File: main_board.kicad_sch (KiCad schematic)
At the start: 21 parts, among them SW1 SW_Push, SW2 SW_Push, U4 QM_XC7A35T_DDR3, U8 XLH536074.250000I

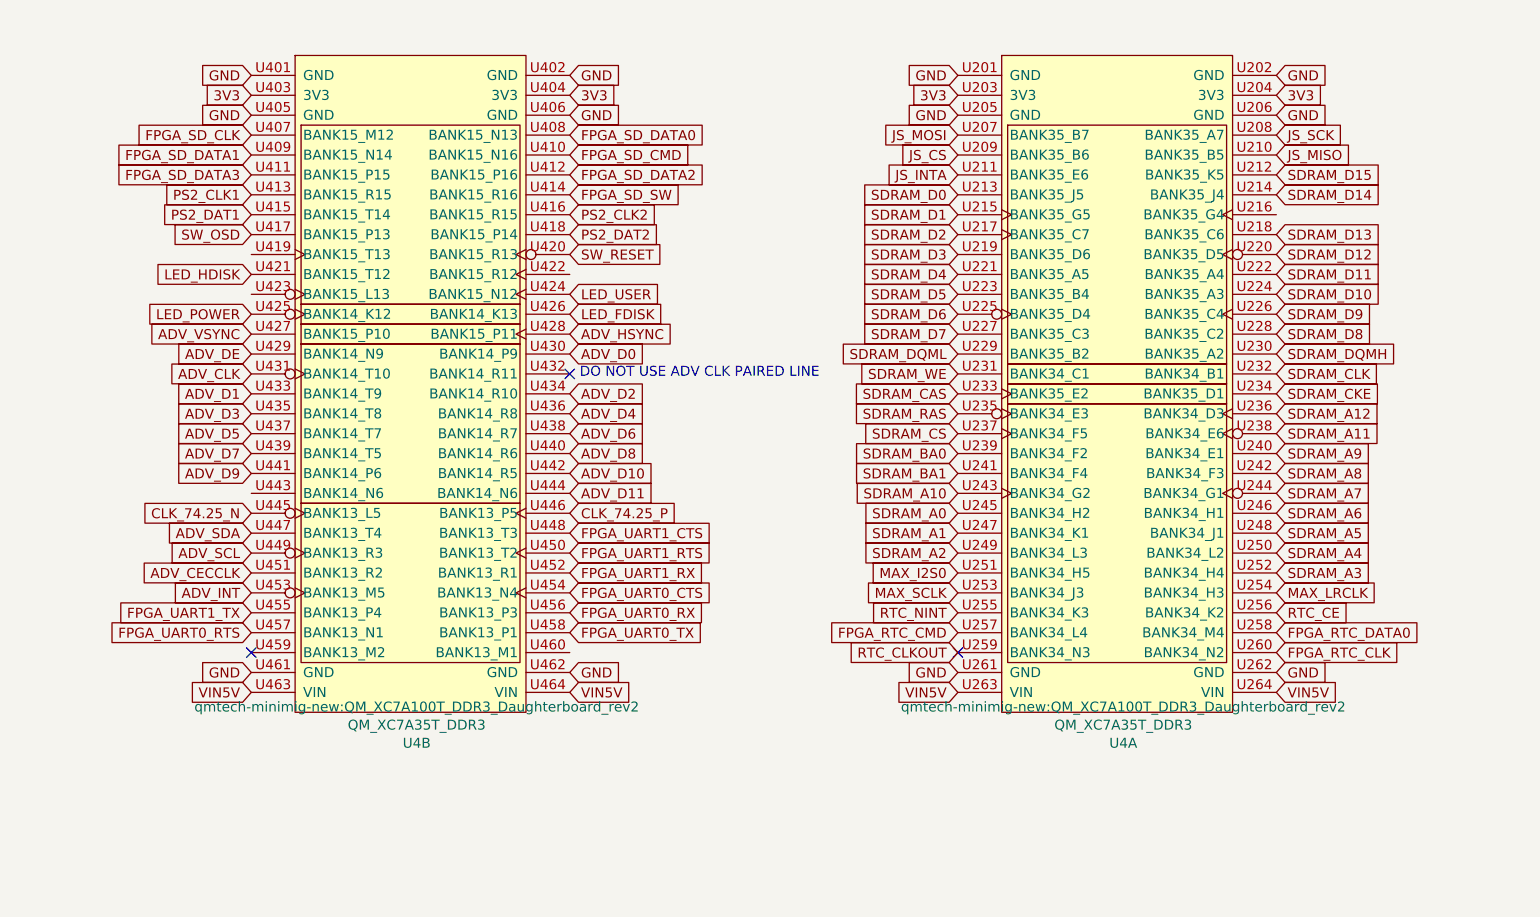
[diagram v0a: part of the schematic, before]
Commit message: V5 Version of the board.
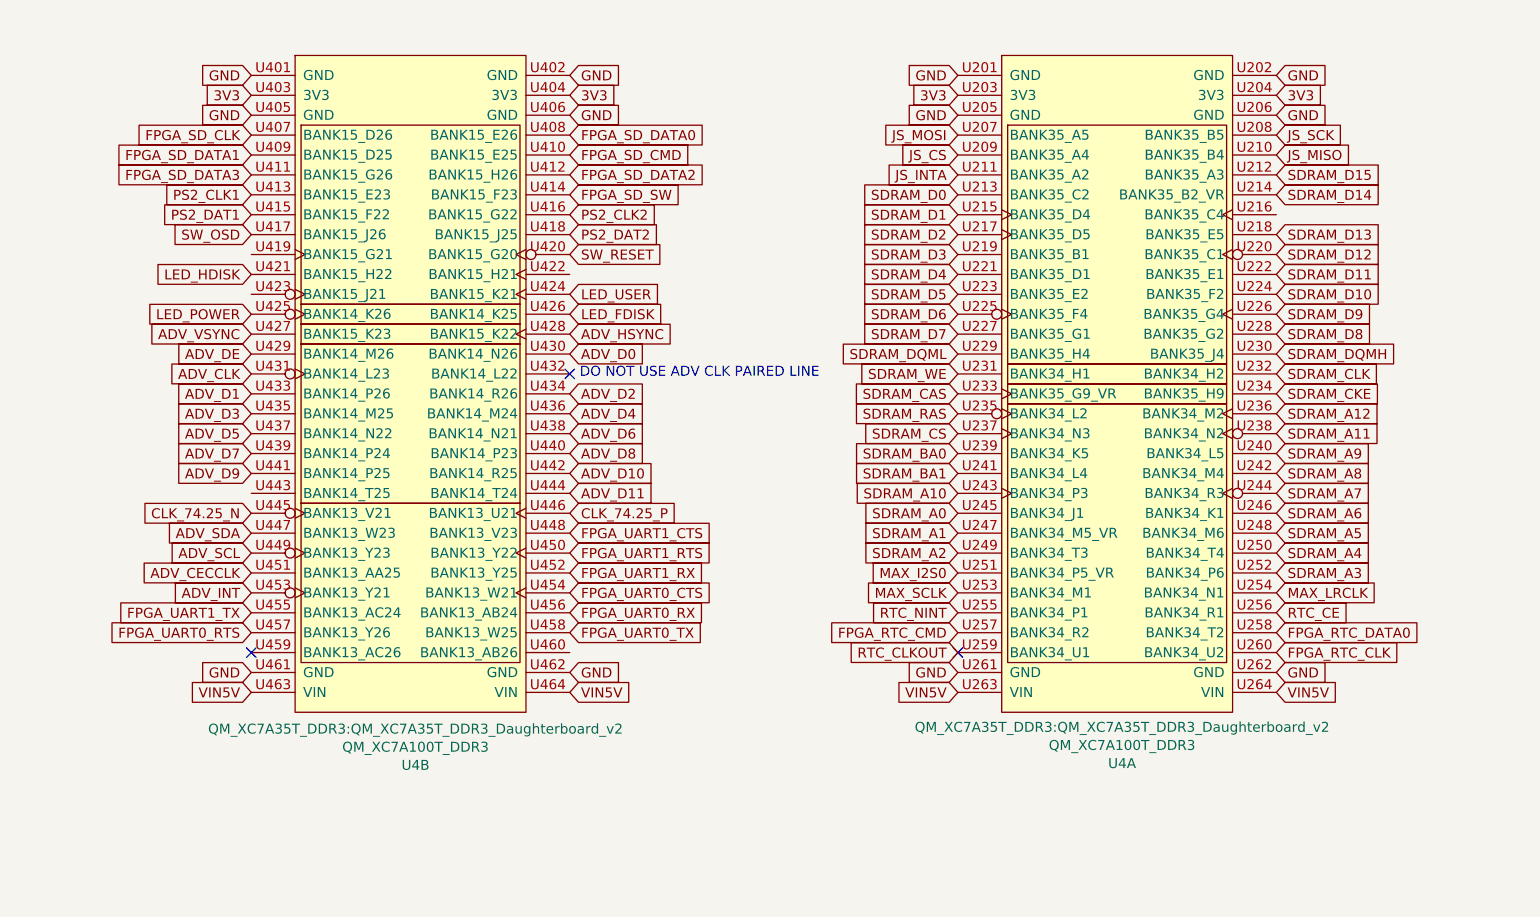
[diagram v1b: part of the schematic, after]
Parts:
- U4: value QM_XC7A35T_DDR3 -> QM_XC7A100T_DDR3; footprint qmtech-minimig-new:QM_XC7A100T_DDR3_Daughterboard_rev2 -> QM_XC7A35T_DDR3:QM_XC7A35T_DDR3_Daughterboard_v2
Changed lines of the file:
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@@
   (symbol (lib_id "QM_XC7A35T_DDR3:QM_XC7A100T_DDR3_2part") (at 156.21 57.785 0) (unit 1)
     (in_bom yes) (on_board yes) (dnp no)
-    (property "Reference" "U4" (at 156.9974 104.902 0)
-      (effects (font (size 1.27 1.27)))
-    )
-    (property "Value" "QM_XC7A35T_DDR3" (at 156.9974 102.5906 0)
-      (effects (font (size 1.27 1.27)))
-    )
-    (property "Footprint" "qmtech-minimig-new:QM_XC7A100T_DDR3_Daughterboard_rev2" (at 156.9974 100.2792 0)
+    (property "Reference" "U4" (at 156.845 107.4928 0)
+      (effects (font (size 1.27 1.27)))
+    )
+    (property "Value" "QM_XC7A100T_DDR3" (at 156.845 105.1814 0)
+      (effects (font (size 1.27 1.27)))
+    )
+    (property "Footprint" "QM_XC7A35T_DDR3:QM_XC7A35T_DDR3_Daughterboard_v2" (at 156.845 102.87 0)
       (effects (font (size 1.27 1.27)))
     )
@@
     )
   )
-  (symbol (lib_name "QM_XC7A100T_DDR3_2part_1") (lib_id "QM_XC7A35T_DDR3:QM_XC7A100T_DDR3_2part") (at 66.04 57.785 0) (unit 2)
-    (in_bom yes) (on_board yes) (dnp no)
-    (property "Reference" "U4" (at 66.8274 104.902 0)
-      (effects (font (size 1.27 1.27)))
-    )
-    (property "Value" "QM_XC7A35T_DDR3" (at 66.8274 102.5906 0)
-      (effects (font (size 1.27 1.27)))
-    )
-    (property "Footprint" "qmtech-minimig-new:QM_XC7A100T_DDR3_Daughterboard_rev2" (at 66.8274 100.2792 0)
-      (effects (font (size 1.27 1.27)))
-    )
+  (symbol (lib_id "QM_XC7A35T_DDR3:QM_XC7A100T_DDR3_2part") (at 66.04 57.785 0) (unit 2)
+    (in_bom yes) (on_board yes) (dnp no)
+    (property "Reference" "U4" (at 66.675 107.7214 0)
+      (effects (font (size 1.27 1.27)))
+    )
+    (property "Value" "QM_XC7A100T_DDR3" (at 66.675 105.41 0)
+      (effects (font (size 1.27 1.27)))
+    )
+    (property "Footprint" "QM_XC7A35T_DDR3:QM_XC7A35T_DDR3_Daughterboard_v2" (at 66.675 103.0986 0)
+      (effects (font (size 1.27 1.27)))
+    )
